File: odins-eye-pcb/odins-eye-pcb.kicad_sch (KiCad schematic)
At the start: 8 parts, among them J1 Conn_01x07_Pin, J2 Conn_01x06_Pin, J3 USB_C_Receptacle_USB2.0_16P, U1 Raspberry Pi Zero 2 W Header

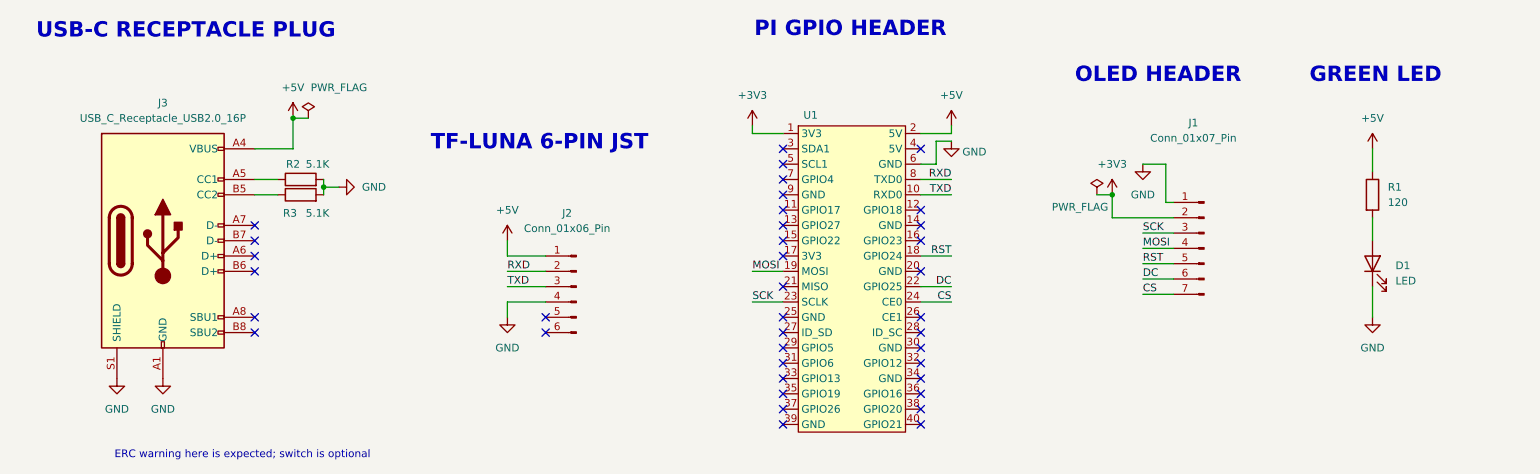
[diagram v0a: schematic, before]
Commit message: Add odins-eye v1.1
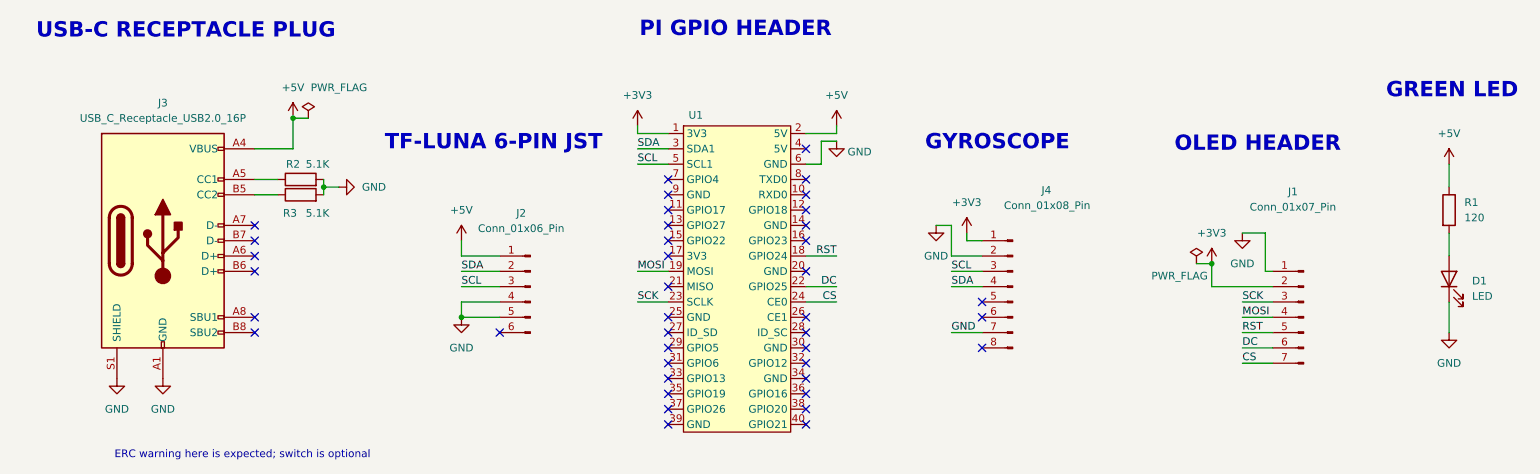
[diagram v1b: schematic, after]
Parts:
- added J4: Conn_01x08_Pin, Connector_PinSocket_2.54mm:PinSocket_1x08_P2.54mm_Vertical, symbol Connector:Conn_01x08_Pin
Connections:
- net +3V3: now also J4.1 (Pin_1)
- net GND: now also J2.5 (Pin_5), J4.2 (Pin_2), J4.7 (Pin_7)
- net SDA: now reaches U1.3 (SDA1)
- net SDA: now also J2.2 (Pin_2), J4.4 (Pin_4)
- net SCL: now reaches U1.5 (SCL1)
- net SCL: now also J2.3 (Pin_3), J4.3 (Pin_3)
- net RXD: no longer names the net of U1.8 (TXD0)
- net RXD: no longer J2.2 (Pin_2)
- net TXD: no longer names the net of U1.10 (RXD0)
- net TXD: no longer J2.3 (Pin_3)
- no-connect marks 38 -> 40
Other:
- note added: "GYROSCOPE"
- moved on the sheet: D1, J1, J2, R1, U1
